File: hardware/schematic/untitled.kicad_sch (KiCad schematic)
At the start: 35 parts, among them J1 Screw_Terminal_01x02, Q1 IRF5210S, U1 LM5164DDA, U2 LM317_SOT-223, U3 AMS1117-3.3

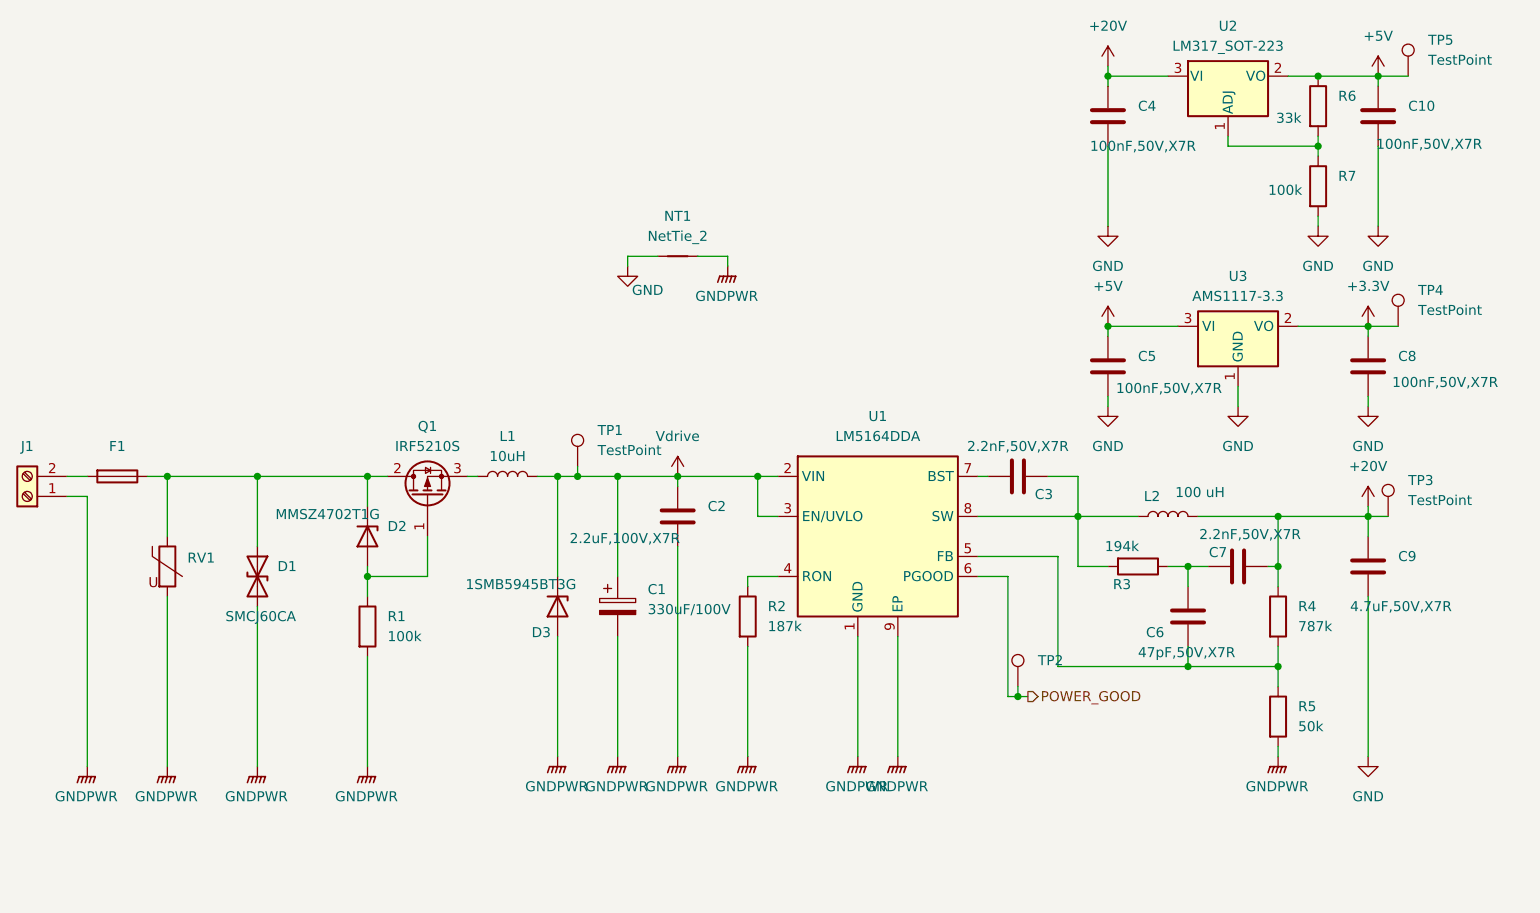
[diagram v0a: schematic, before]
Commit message: pcb improvements
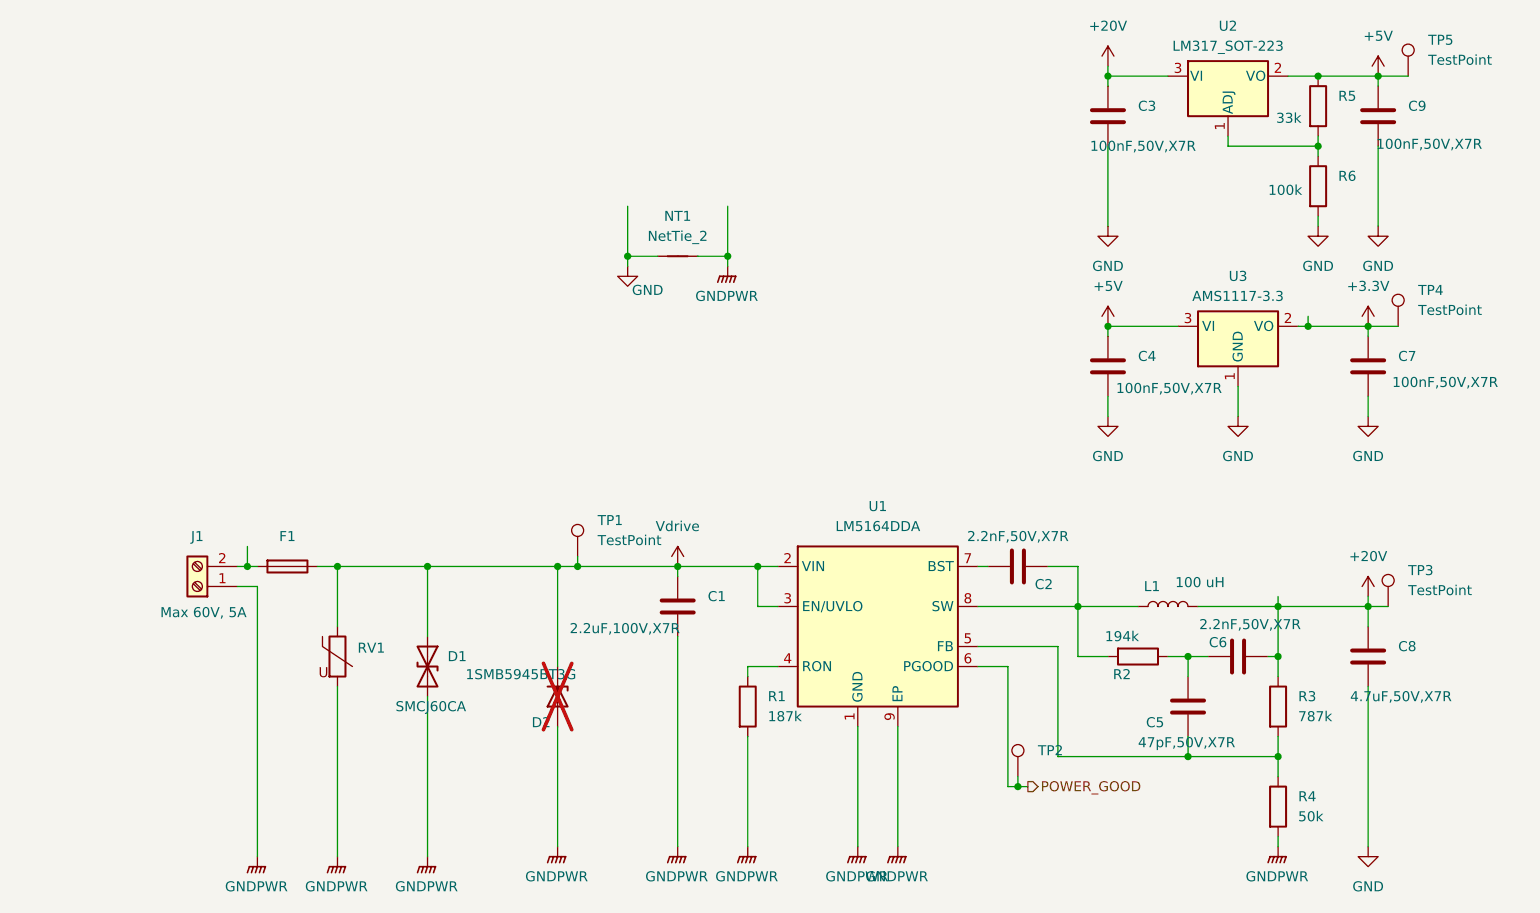
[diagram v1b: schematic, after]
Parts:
- removed C1: 330uF/100V, Capacitor_SMD:CP_Elec_18x22, symbol Device:C_Polarized
- removed D2: MMSZ4702T1G, Diode_SMD:D_SOD-123, symbol Device:D_Zener
- removed L1: 10uH, Inductor_SMD:L_12x12mm_H8mm, symbol Device:L
- removed Q1: IRF5210S, Package_TO_SOT_SMD:TO-263-2, symbol Transistor_FET:Q_PMOS_GDS
- removed R1: 100k, Resistor_SMD:R_0805_2012Metric_Pad1.20x1.40mm_HandSolder, symbol Device:R
- C1: renamed from C2; footprint (none) -> Capacitor_SMD:C_0805_2012Metric_Pad1.18x1.45mm_HandSolder
- C2: renamed from C3; footprint (none) -> Capacitor_SMD:C_0805_2012Metric_Pad1.18x1.45mm_HandSolder
- C3: renamed from C4; footprint (none) -> Capacitor_SMD:C_0805_2012Metric_Pad1.18x1.45mm_HandSolder
- C4: renamed from C5; footprint (none) -> Capacitor_SMD:C_0805_2012Metric_Pad1.18x1.45mm_HandSolder
- C5: renamed from C6; footprint (none) -> Capacitor_SMD:C_0805_2012Metric_Pad1.18x1.45mm_HandSolder
- C6: renamed from C7; footprint (none) -> Capacitor_SMD:C_0805_2012Metric_Pad1.18x1.45mm_HandSolder
- C7: renamed from C8; footprint (none) -> Capacitor_SMD:C_0805_2012Metric_Pad1.18x1.45mm_HandSolder
- C8: renamed from C9; footprint (none) -> Capacitor_SMD:C_0805_2012Metric_Pad1.18x1.45mm_HandSolder
- C9: renamed from C10; footprint (none) -> Capacitor_SMD:C_0805_2012Metric_Pad1.18x1.45mm_HandSolder
- D2: renamed from D3; now not fitted
- J1: footprint TerminalBlock:TerminalBlock_Xinya_XY308-2.54-2P_1x02_P2.54mm_Horizontal -> TerminalBlock_CUI:TerminalBlock_CUI_TB007-508-02_1x02_P5.08mm_Horizontal; Usage (none) -> Max 60V, 5A
- L1: renamed from L2; footprint Inductor_SMD:L_12x12mm_H8mm -> Inductor_SMD:L_7.3x7.3_H4.5
- renumbered R2 to R1, R3 to R2, R4 to R3, R5 to R4, R6 to R5, R7 to R6
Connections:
- net Vdrive: now also D1.1 (A1), F1.1, RV1.1
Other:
- moved on the sheet: C1, C2, C5, C6, C8, D1, F1, J1, L1, R1, R2, R3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

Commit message: board finished
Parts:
- U1: footprint Package_SO:HSOP-8-1EP_3.9x4.9mm_P1.27mm_EP2.41x3.1mm_ThermalVias -> Package_SO:HSOP-8-1EP_3.9x4.9mm_P1.27mm_EP2.41x3.1mm
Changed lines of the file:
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@@
 			)
 		)
-		(property "Footprint" "Package_SO:HSOP-8-1EP_3.9x4.9mm_P1.27mm_EP2.41x3.1mm_ThermalVias"
+		(property "Footprint" "Package_SO:HSOP-8-1EP_3.9x4.9mm_P1.27mm_EP2.41x3.1mm"
 			(at 172.72 128.27 0)
 			(hide yes)
